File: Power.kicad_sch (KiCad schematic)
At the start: 28 parts, among them Q3 AO3400A, Q4 AO3400A, Q6 AO3401, U11 TLV809I50, U13 MAX40200AUK, U14 BQ21040DBVR, U15 BQ297xxDSE, U8 XC6206P332MR

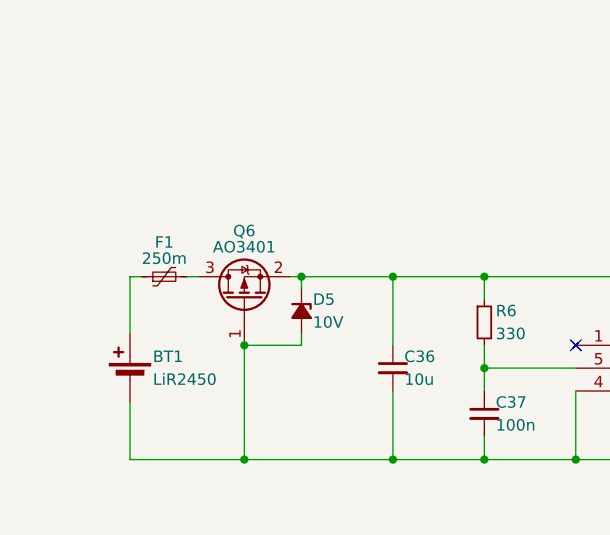
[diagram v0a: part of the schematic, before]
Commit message: idk
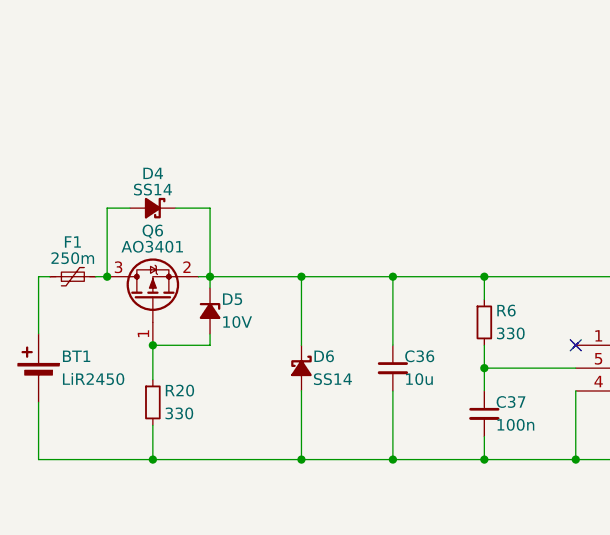
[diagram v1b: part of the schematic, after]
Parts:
- added D4, D6: SS14, symbol Device:D_Schottky_Small_Filled
- added R20: 330, symbol Device:R_Small
- D5: footprint (none) -> stdpads:D_SOD-323
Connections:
- net at C36.1, D5.1 (K), Q6.2 (S)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: now also D4.1 (K), D6.1 (K)
- net at BT1.2 (-), C36.2, C37.2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: now also D6.2 (A), R20.2; no longer D5.2 (A), Q6.1 (G)
- net at F1.2, Q6.3 (D): now also D4.2 (A)
- new net: D5.2 (A), Q6.1 (G), R20.1
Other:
- moved on the sheet: BT1, D5, F1, Q6
